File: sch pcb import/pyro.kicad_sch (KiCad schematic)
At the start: 22 parts, among them J601 Screw_Terminal_01x04, Q601 SISA12ADN, Q602 SISA12ADN, U601 LM358

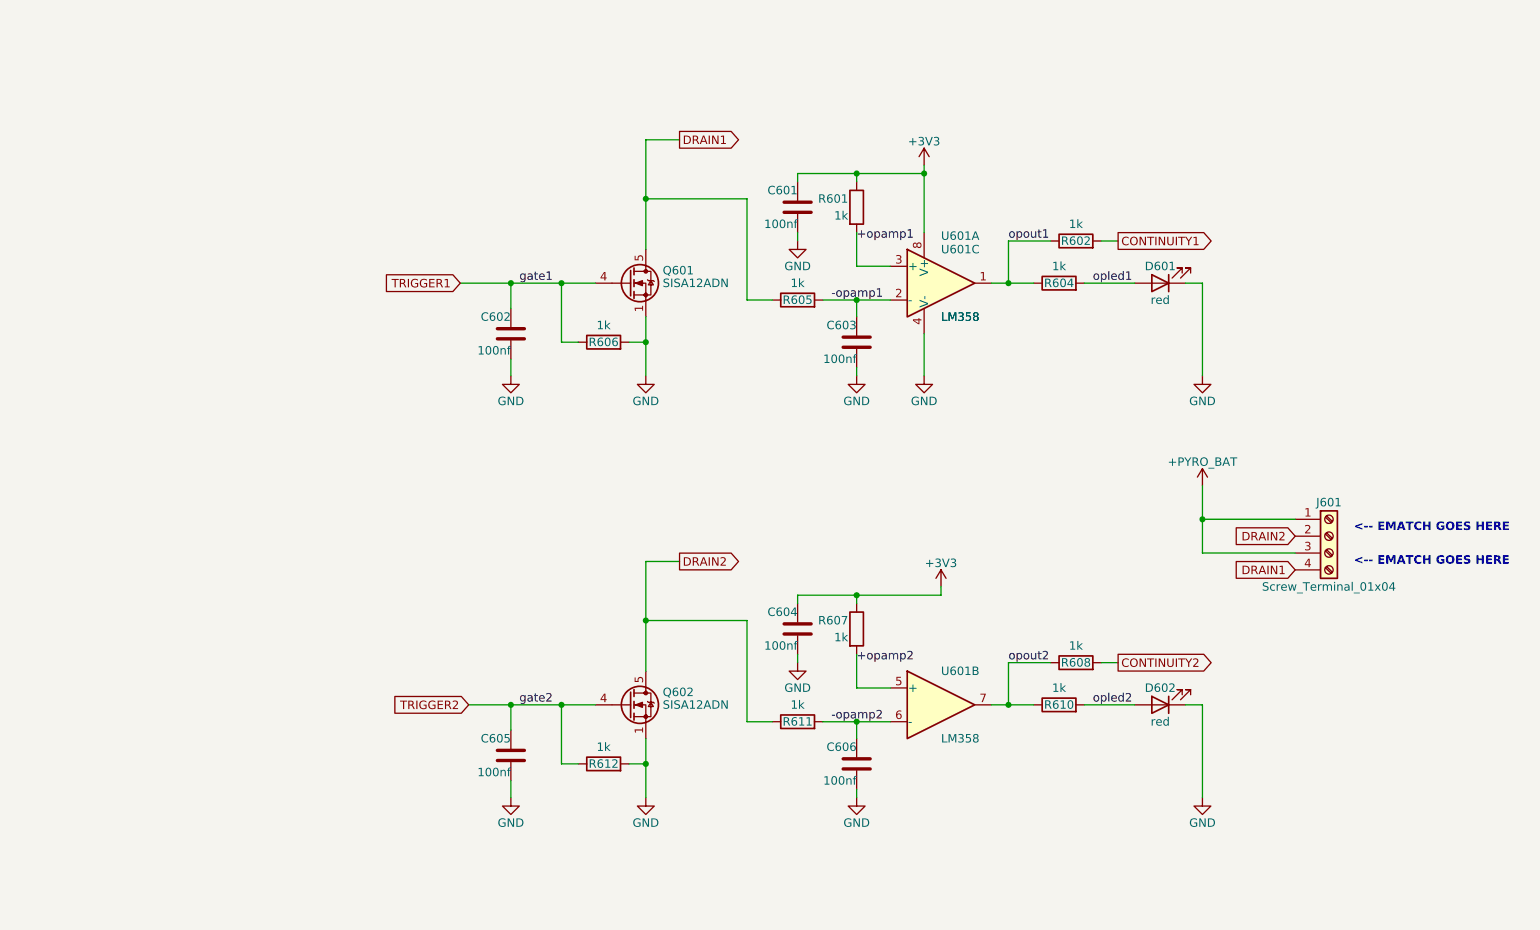
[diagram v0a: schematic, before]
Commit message: rearranging for aesthetics
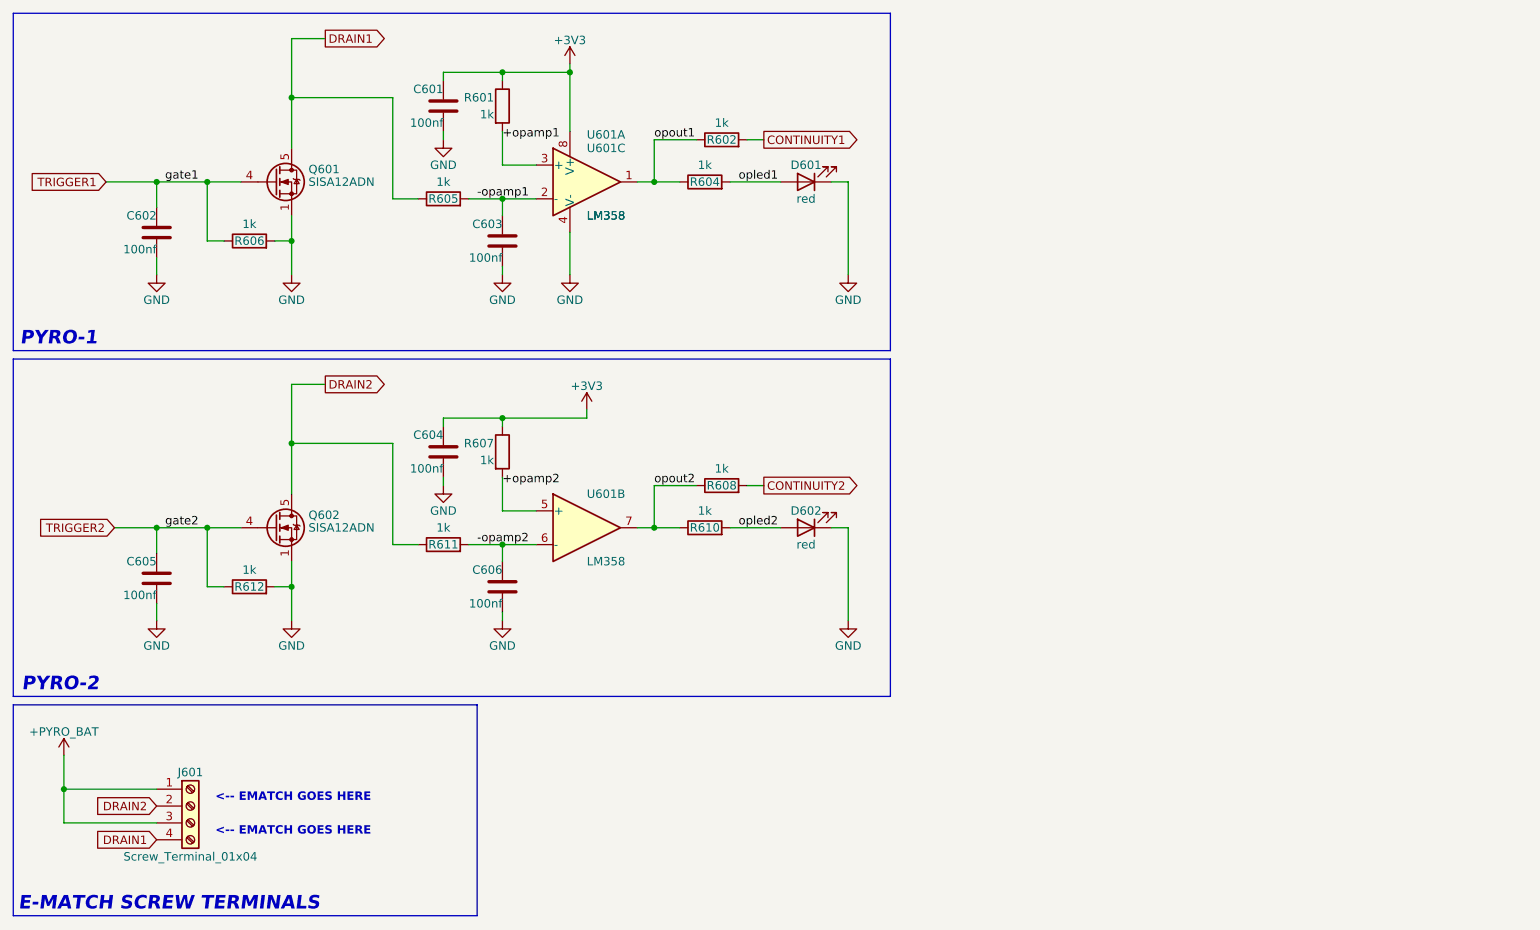
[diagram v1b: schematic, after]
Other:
- note added: "E-MATCH SCREW TERMINALS"
- note added: "PYRO-1"
- note added: "PYRO-2"
- moved on the sheet: C601, C602, C603, C604, C605, C606, D601, D602, J601, Q601, Q602, R601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
